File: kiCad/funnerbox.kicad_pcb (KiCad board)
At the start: 2 copper layers, 59.7 x 67.5 mm, 48 parts, among them J6 MIDI IN, J7 EXPRESSION, SW1 SW_SPDT, SW2 SW_SPDT, U1 MCP6024, U2 L7805, U3 MCP6002, U5 H11L1

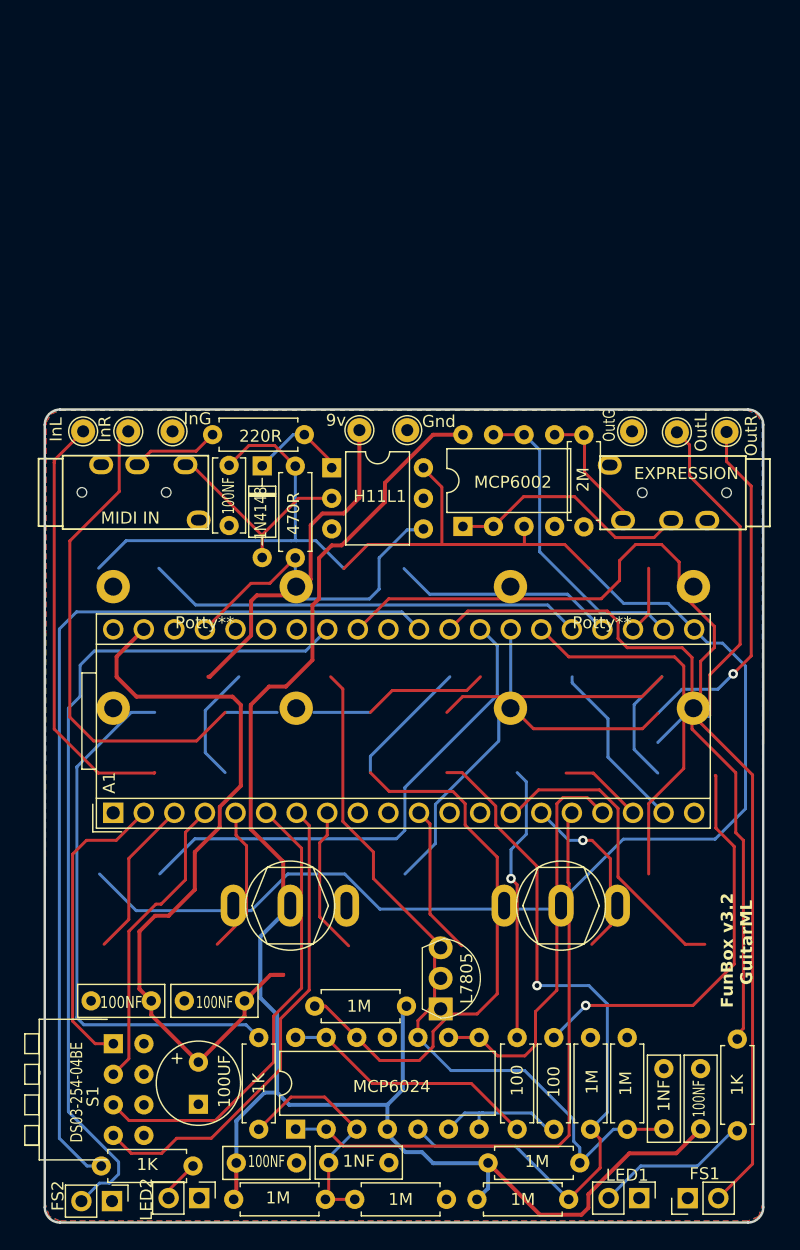
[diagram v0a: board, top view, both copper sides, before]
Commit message: Lots of stuff
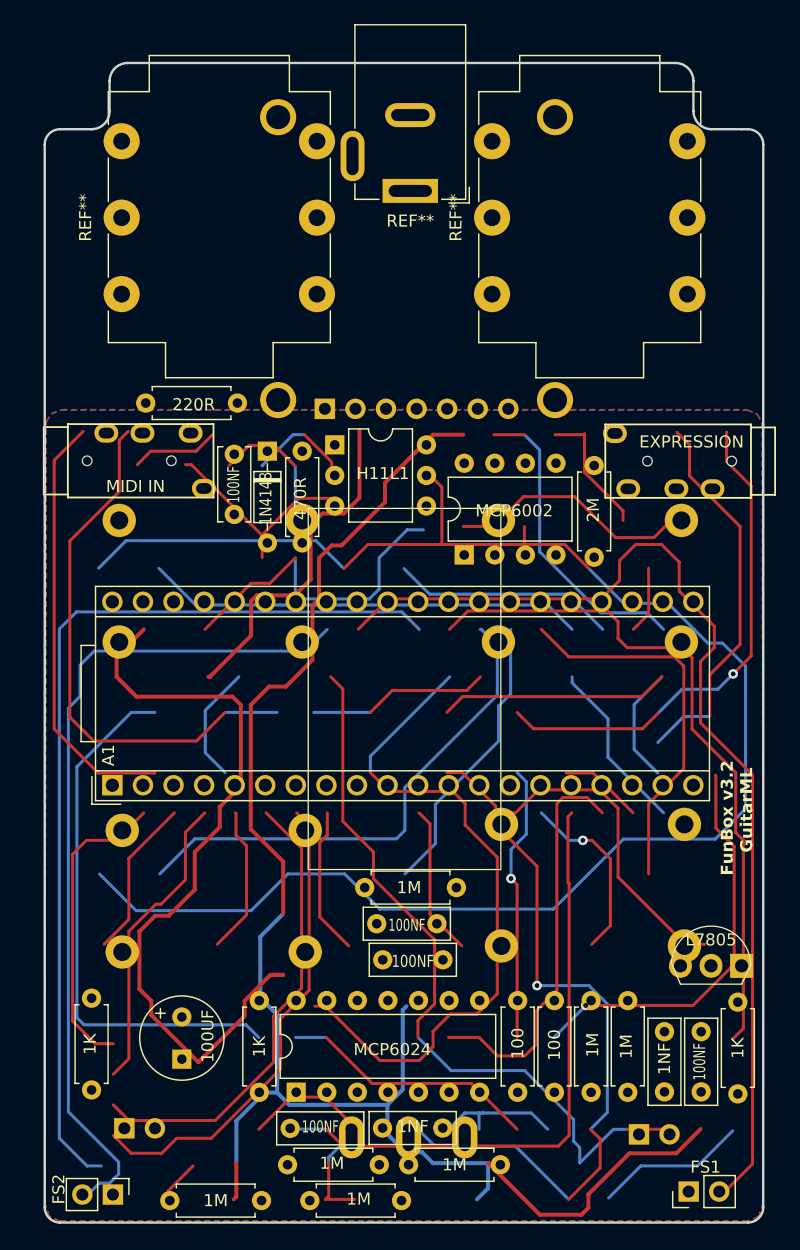
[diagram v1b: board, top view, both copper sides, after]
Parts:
- removed 9v, Gnd, InG, InL, InR, OutG, OutL, OutR: ~, TestPoint:TestPoint_THTPad_D2.0mm_Drill1.0mm
- removed S1: DS03-254-04BE, Button_Switch_THT:DS03-254-04BE-dip4
- removed SW1: SW_SPDT, Button_Switch_THT:SW_Toggle_SPDT_lugs
- added Potty**: Potty, Custom_FP:Potty, B.Cu at (131.9, 78.5)
- added Potty**: Potty, Custom_FP:Potty, B.Cu at (163.4, 78.5)
- added REF**: Jack_6.35mm_Neutrik_NMJ6HCD2_Horizontal, Connector_Audio:Jack_6.35mm_Neutrik_NMJ6HCD2_Horizontal, F.Cu at (124.5, 54.7)
- added REF**: Jack_6.35mm_Neutrik_NMJ6HCD2_Horizontal, Connector_Audio:Jack_6.35mm_Neutrik_NMJ6HCD2_Horizontal, F.Cu at (155.3, 54.7)
- added REF**: BarrelJack_GCT_DCJ200-10-A_Horizontal, Connector_BarrelJack:BarrelJack_GCT_DCJ200-10-A_Horizontal, F.Cu at (148.5, 46.1)
- added REF**: Enclosure, Custom_FP:Enclosure, F.Cu at (148.0, 93.0)
- added REF**: HiLetgo_OLED_SPI, CustomFootprints:HiLetgo_OLED_SPI, B.Cu at (149.0, 52.0)
- LED1, LED2, Potty** (x2), SW2: moved to B.Cu
- moved R5 25.5 mm to (128.5, 130.0)
- moved U2 25.3 mm to (176.0, 110.5), turned to 180 degrees
- moved C8 24.5 mm to (146.2, 110.0)
- moved SW2 21.6 mm to (148.3, 124.8)
- moved Potty** 20.3 mm to (132.2, 104.2), turned to 180 degrees
- moved Potty** 19.8 mm to (163.7, 103.8), turned to 180 degrees
- moved C7 17.2 mm to (145.7, 107.0)
- moved R9 16.3 mm to (122.0, 113.2), turned to -90 degrees
- moved R15 15.1 mm to (140.1, 130.0)
- moved R13 10.7 mm to (152.3, 104.0)
- moved LED2 8.50 mm to (124.7, 124.0)
- moved R30 6.14 mm to (126.5, 63.8)
- moved C3 5.32 mm to (151.2, 124.0)
- moved C9 5.32 mm to (143.5, 124.0)
- moved R1 5.32 mm to (148.3, 127.0)
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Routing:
- net GND: track 0.00 -> 144.6 mm, vias 0 -> 2
- net 3V3_A: track 154.9 -> 28.5 mm
- net VCC: track 63.6 -> 155.2 mm
- net Net-(U1D-+): track 45.9 -> 135.0 mm
- net SW2_LEFT: track 12.3 -> 90.1 mm
- net LED_2: track 77.8 -> 0.00 mm
- net Net-(U1C-+): track 61.8 -> 0.00 mm
- net POT_5: track 55.8 -> 0.00 mm
- net Net-(C1-Pad2): track 45.0 -> 0.00 mm
- net unconnected-(A1-I2C1_SCL-Pad12): track 0.00 -> 42.4 mm
- net SW1_LEFT: track 15.1 -> 57.1 mm, vias 1 -> 0
- net POT_3: track 36.4 -> 0.00 mm
- net 3V3_D: track 0.00 -> 36.4 mm
- net AUDIO_IN_BUFFER_RIGHT: track 33.6 -> 0.00 mm
- net Net-(Out1-Pin_1): track 32.0 -> 0.00 mm
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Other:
- board size 59.7 x 67.5 mm -> 59.7 x 96.3 mm
